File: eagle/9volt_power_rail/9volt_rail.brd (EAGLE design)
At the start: 94.9 x 67.3 mm, 48 parts, among them IC1 TL331

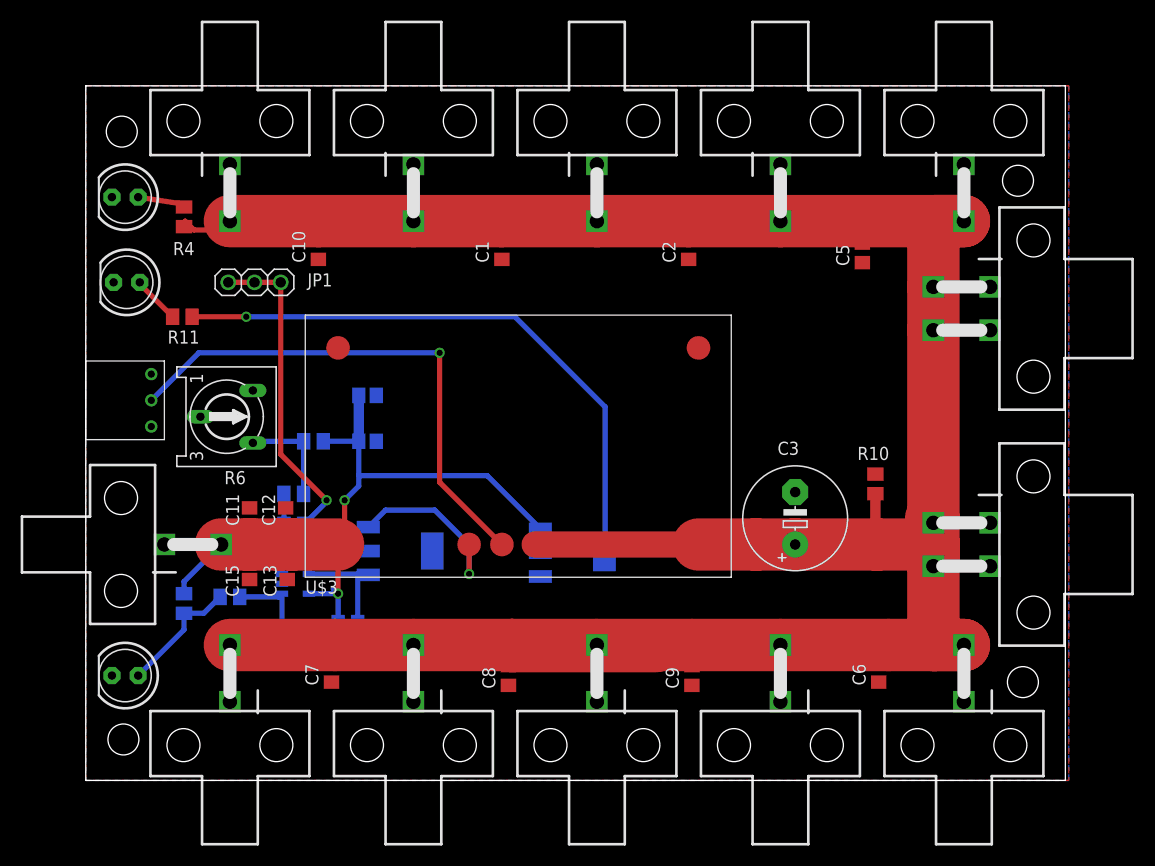
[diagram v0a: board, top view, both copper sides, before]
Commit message: Done with power board and adc cape
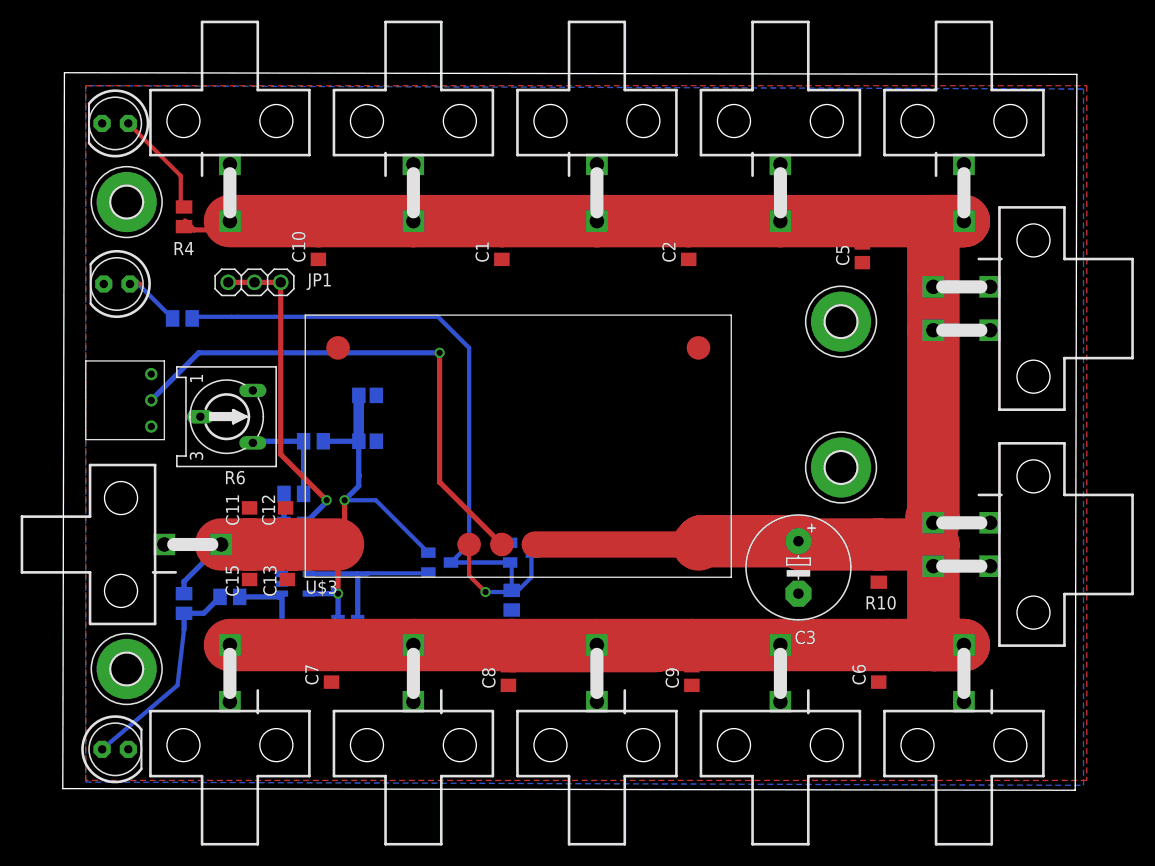
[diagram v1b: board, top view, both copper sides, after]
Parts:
- removed T1, T3: (no value), zetex:SOT223
- added H1, H2, H3, H4: MOUNT-PAD-ROUND3.0, holes:3,0-PAD
- added Q1: BSS84, transistor-small-signal:SOT23
- added Q2: BSS123, transistor-small-signal:SOT23
- added R12: (no value), adafruit:M0805
- moved R10 8.58 mm to (75.6, 20.2), turned to 270 degrees
- moved VCC1 7.21 mm to (1.59, 3.02), turned to 0 degrees
- moved VCC2 7.21 mm to (1.59, 63.7)
- moved C3 4.77 mm to (67.8, 20.6), turned to 270 degrees
- moved VCC3 0.97 mm to (1.75, 48.1)
- moved R11 0.16 mm to (8.10, 44.8), flipped to the bottom, turned to 0 degrees
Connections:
- net GND: now also H1.B3,0, H2.B3,0, H3.B3,0, H4.B3,0, Q2.2, R12.2; no longer T3.2, T3.4
- net N$10: now also Q2.3, U$3.3; no longer R11.1, T1.2, T1.4
- net N$2: now also Q1.1; no longer T1.1, T3.1
- net N$5: now also Q1.3, Q2.1, R11.1, R12.1; no longer T3.3, U$3.3
- net VCC: now also Q1.2; no longer T1.3
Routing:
- net N$10: track 64.0 -> 12.7 mm
- net N$5: track 17.5 -> 58.2 mm, vias 1 -> 0
- net VCC: track 75.2 -> 65.7 mm
- net N$3: track 12.0 -> 20.8 mm
- net N$2: track 47.1 -> 53.1 mm
- net N$9: track 4.63 -> 10.3 mm
- net N$8: track 4.65 -> 6.46 mm
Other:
- board size 94.9 x 67.3 mm -> 98.3 x 69.5 mm
